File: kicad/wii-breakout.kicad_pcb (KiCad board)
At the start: 2 copper layers, 12.6 x 69.8 mm, 11 parts, among them J1 Peripherals, J2 Audio, J3 Video, J4 USB, J5 GC, J6 Rst, J7 BT, J8 Audio, J9 Video

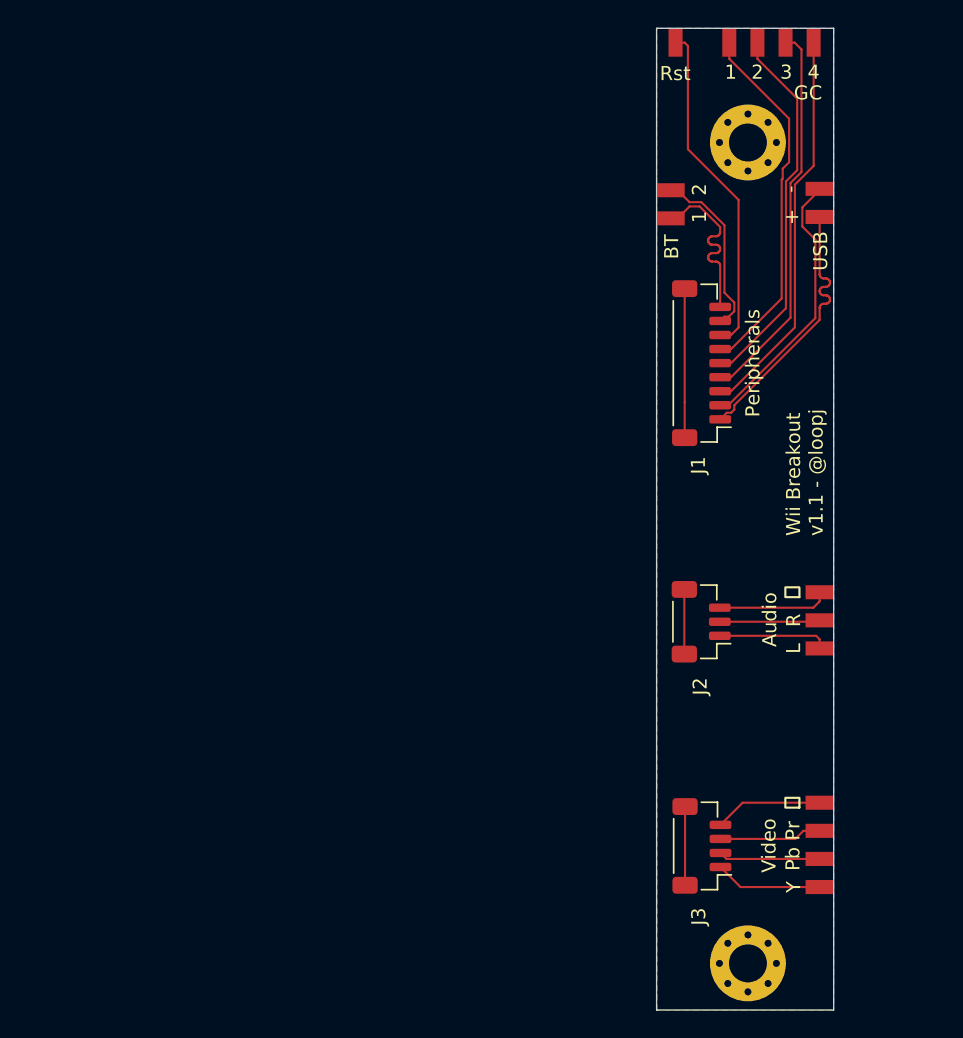
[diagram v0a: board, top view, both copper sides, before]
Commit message: v2.0
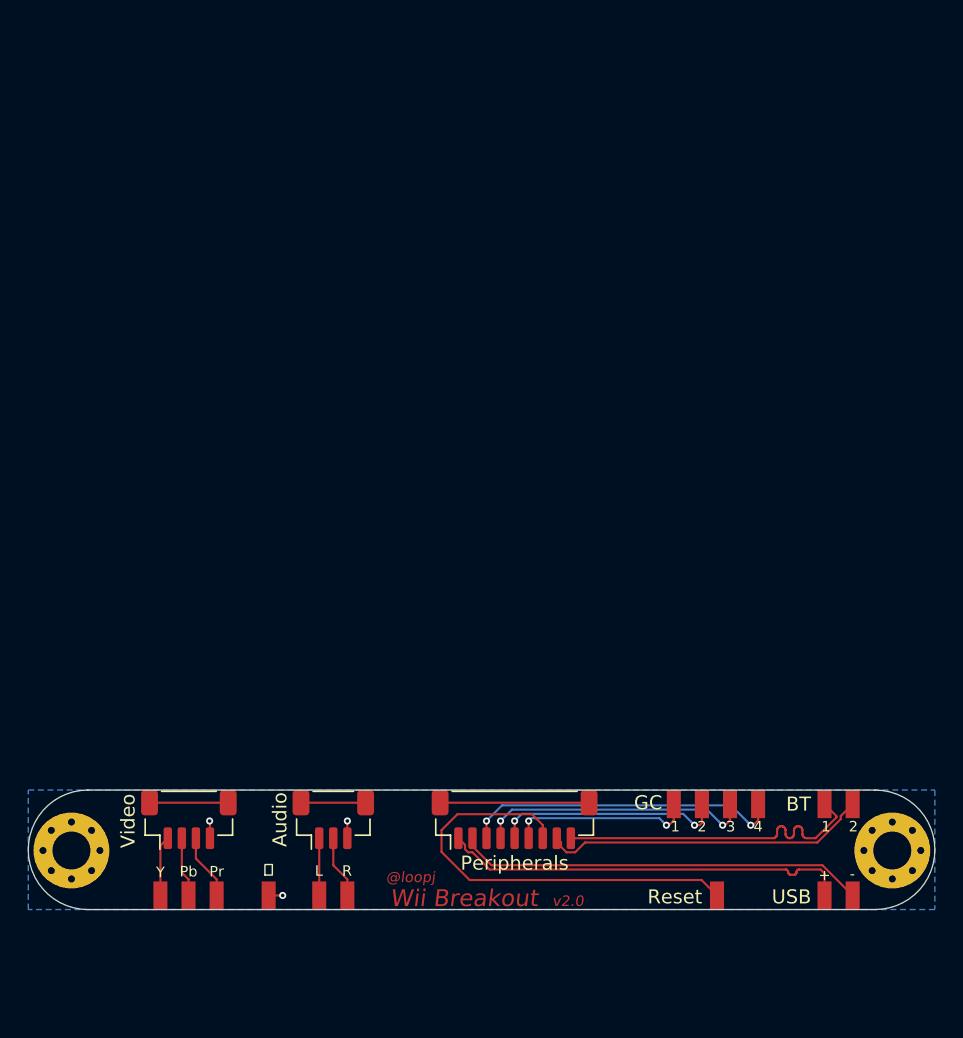
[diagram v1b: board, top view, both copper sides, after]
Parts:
- added J10: ⏚, project-footprints:TestPoint_Pad_2.0x1.0mm, F.Cu at (49.0, 107.6)
- J4, J7: footprint TestPoint:TestPoint_2Pads_2.0x1.0mm -> project-footprints:TestPoint_2Pads_2.0x1.0mm
- J5: footprint TestPoint:TestPoint_4Pads_2.0x1.0mm -> project-footprints:TestPoint_4Pads_2.0x1.0mm
- J6: value Rst -> Reset; footprint TestPoint:TestPoint_Pad_2.0x1.0mm -> project-footprints:TestPoint_Pad_2.0x1.0mm
- J8: footprint TestPoint:TestPoint_3Pads_2.0x1.0mm -> project-footprints:TestPoint_2Pads_2.0x1.0mm
- J9: footprint TestPoint:TestPoint_4Pads_2.0x1.0mm -> project-footprints:TestPoint_3Pads_2.0x1.0mm
- moved J6 60.7 mm to (80.9, 107.6), turned to 90 degrees
- moved J5 54.3 mm to (80.8, 101.1)
- moved H1 51.4 mm to (93.4, 104.4), turned to 270 degrees
- moved J4 49.3 mm to (89.5, 107.6), turned to 90 degrees
- moved H2 48.8 mm to (35.0, 104.4), turned to 270 degrees
- moved J9 45.0 mm to (43.3, 107.6), turned to 90 degrees
- moved J7 44.3 mm to (89.5, 101.1), turned to 270 degrees
- moved J8 39.8 mm to (53.6, 107.6), turned to 90 degrees
- moved J3 36.5 mm to (43.3, 102.2), turned to 0 degrees
- moved J1 35.1 mm to (66.5, 102.2), turned to 0 degrees
- moved J2 29.7 mm to (53.6, 102.2), turned to 0 degrees
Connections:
- J2 pad 3: /AUDIO_GND -> GND
- J3 pad 4: /VIDEO_GND -> GND
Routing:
- net /GC_1: track 26.0 -> 13.1 mm, vias 0 -> 2
- net /BT_D-: track 12.6 -> 23.2 mm
- net /BT_D+: track 12.6 -> 23.2 mm
- net /GC_2: track 26.7 -> 16.5 mm, vias 0 -> 2
- net /USB_D+: track 19.4 -> 29.3 mm
- net /USB_D-: track 19.4 -> 29.1 mm
- net /AUDIO_GND: track 7.94 -> 0.00 mm
- net /GC_3: track 27.5 -> 19.6 mm, vias 0 -> 2
- net /VIDEO_GND: track 7.70 -> 0.00 mm
- net /RST: track 24.0 -> 31.4 mm
- net /GC_4: track 28.0 -> 22.9 mm, vias 0 -> 2
- net /AUDIO_LEFT: track 7.85 -> 4.07 mm
- net GND: track 0.00 -> 3.46 mm, vias 0 -> 3
- net /VIDEO_Y: track 7.64 -> 4.29 mm
- net /VIDEO_PB: track 7.23 -> 4.27 mm
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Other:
- board size 12.6 x 69.8 mm -> 64.5 x 8.5 mm
- board text added: "@loopj"
- board text added: "Wii Breakout"
- board text added: "v2.0"
- board text removed: "Wii Breakout v1.1 - @loopj"
- board text removed: "⏚"
